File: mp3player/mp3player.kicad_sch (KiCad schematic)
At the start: 9 parts, among them J1 OLED_128x32, U1 DFR0299, U2 Arduino_Pro_Micro

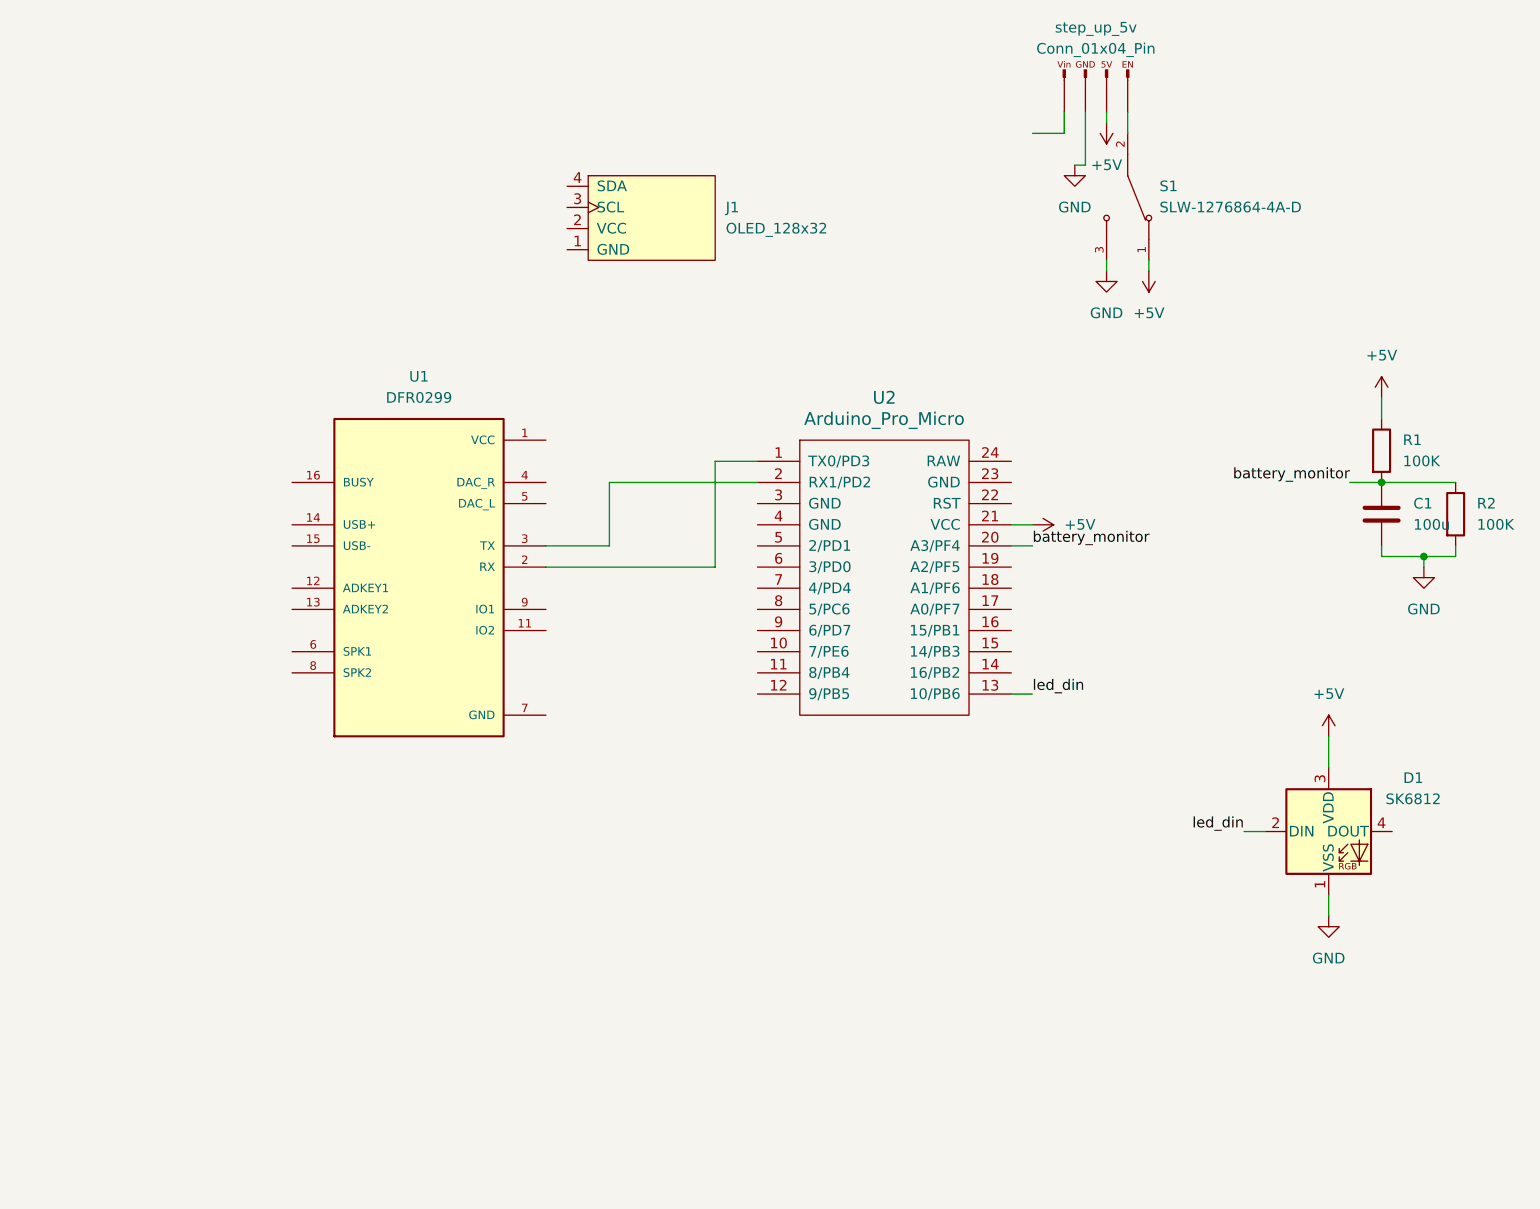
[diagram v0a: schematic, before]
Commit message: ricey
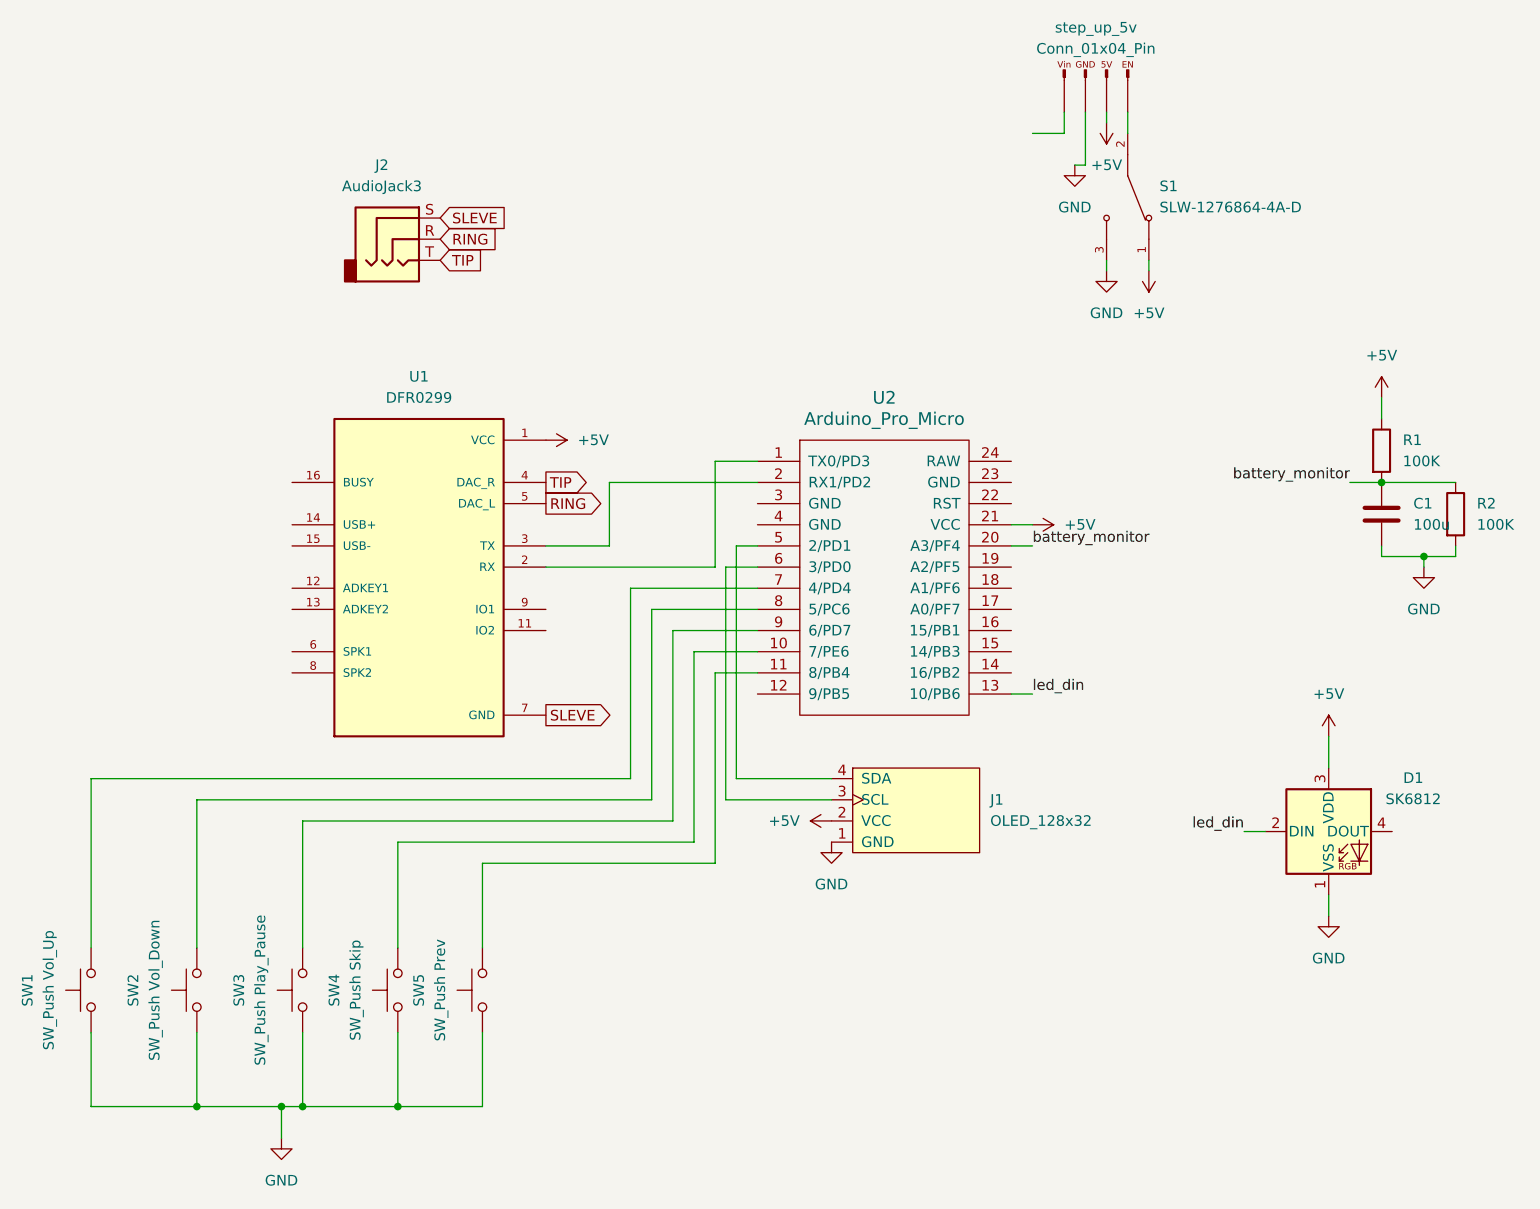
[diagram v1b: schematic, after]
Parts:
- added J2: AudioJack3, symbol Connector_Audio:AudioJack3
- added SW1: SW_Push Vol_Up, symbol Switch:SW_Push
- added SW2: SW_Push Vol_Down, symbol Switch:SW_Push
- added SW3: SW_Push Play_Pause, symbol Switch:SW_Push
- added SW4: SW_Push Skip, symbol Switch:SW_Push
- added SW5: SW_Push Prev, symbol Switch:SW_Push
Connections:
- net +5V: now also J1.2 (VCC), U1.1 (VCC)
- net GND: now also J1.1 (GND), J2.S, SW1.1, SW2.1, SW3.1, SW4.1, SW5.1
- net at J1.3 (SCL): now also U2.6 (3/PD0)
- net at J1.4 (SDA): now also U2.5 (2/PD1)
- net at U2.10 (7/PE6): now also SW4.2
- net at U2.11 (8/PB4): now also SW5.2
- net at U2.7 (4/PD4): now also SW1.2
- net at U2.8 (5/PC6): now also SW2.2
- net at U2.9 (6/PD7): now also SW3.2
- net TIP: now reaches U1.4 (DAC_R)
- net TIP: now also J2.T
- net RING: now reaches U1.5 (DAC_L)
- net RING: now also J2.R
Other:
- moved on the sheet: J1
